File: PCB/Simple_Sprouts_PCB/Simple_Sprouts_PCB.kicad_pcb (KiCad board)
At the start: 4 copper layers, 69 x 70.6 mm, 43 parts, among them J1 Raspberry_Pi_5, J3 Soil Sensor, J4 Soil Sensor, J6 Temperature Sensor, J7 Air Quality Sensor, J8 Humidity Sensor, J9 HC-SR04, Q1 IRLB8721PbF, Q2 IRLB8721PbF, Q3 IRLB8721PbF, Q4 IRLB8721PbF, Q5 IRLB8721PbF, Q6 IRLB8721PbF

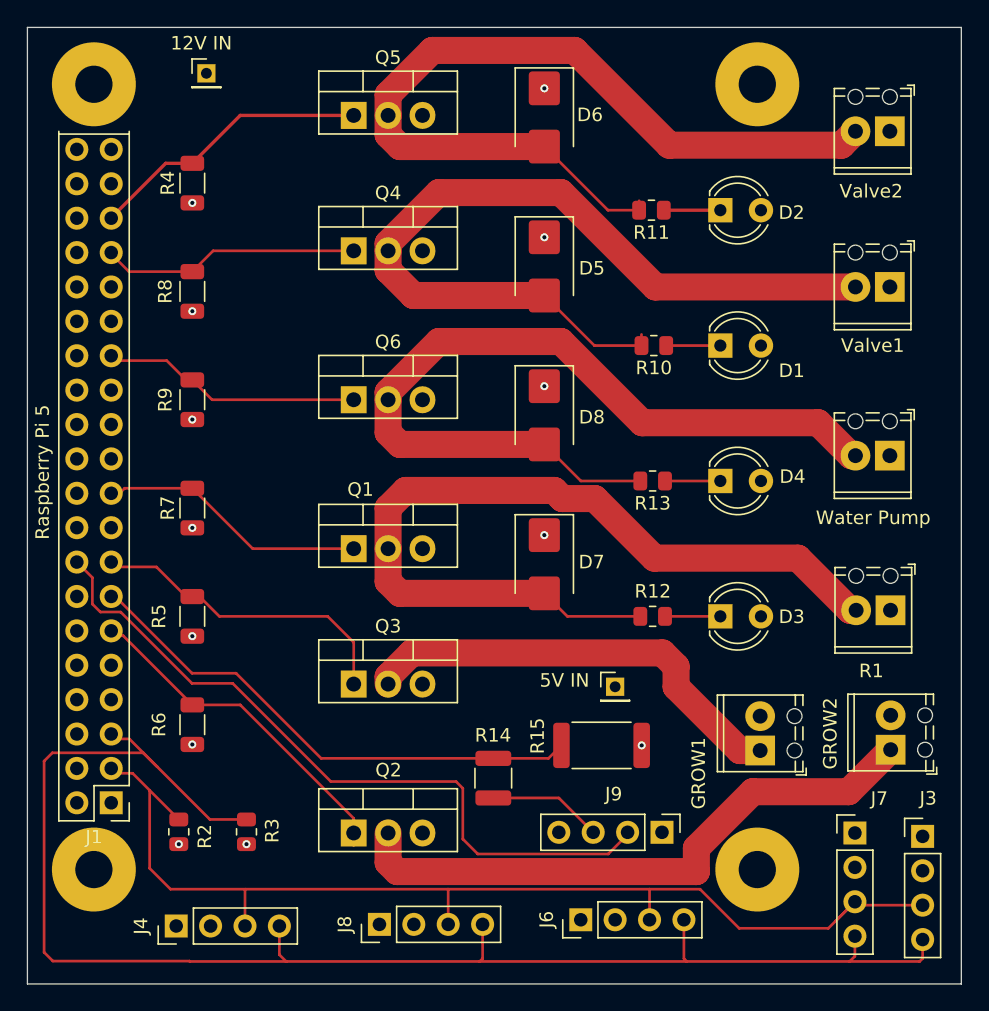
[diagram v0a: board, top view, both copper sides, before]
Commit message: Add files via upload
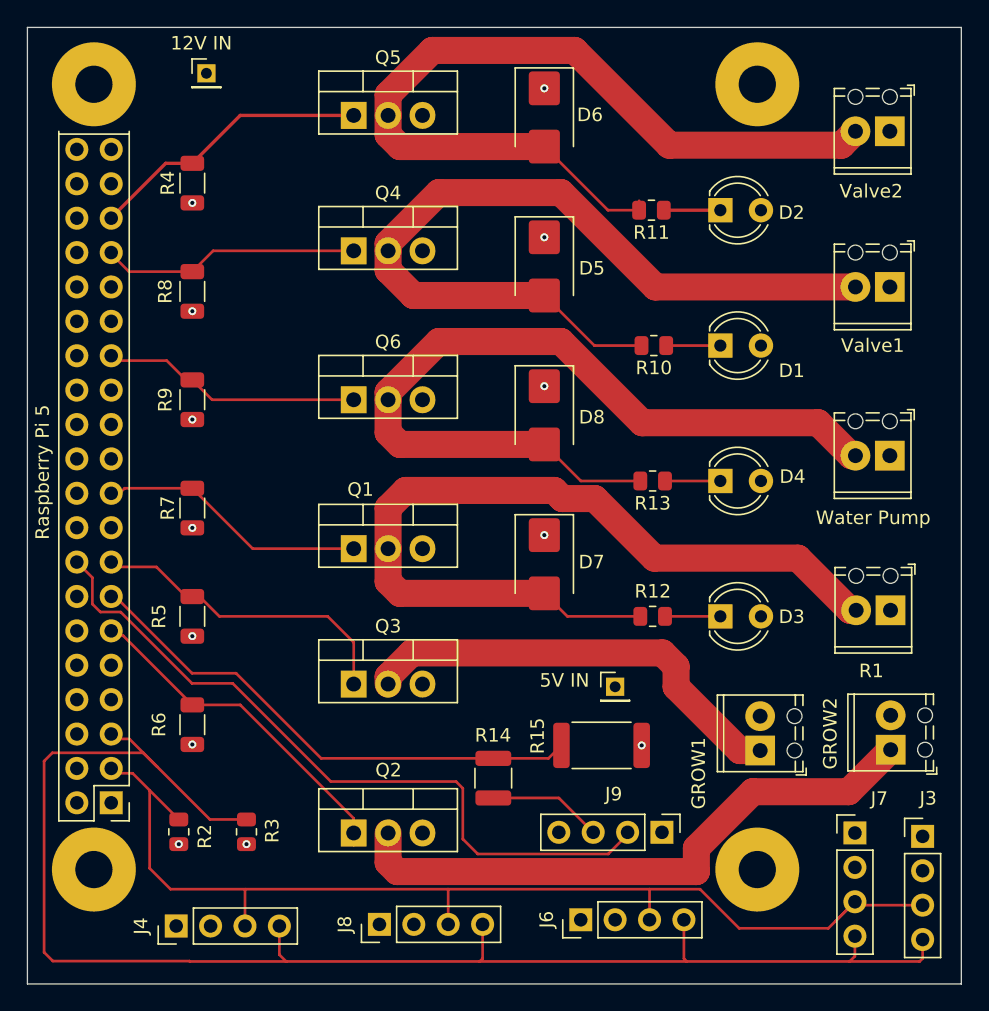
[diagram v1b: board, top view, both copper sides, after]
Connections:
- GROW1 pad 1: (no net) -> Net-(Q3-D)
- GROW1 pad 2: (no net) -> +5V
- GROW2 pad 1: (no net) -> Net-(Q2-D)
- GROW2 pad 2: (no net) -> +5V
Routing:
- net +3.3V: track 11.1 -> 34.4 mm
- net +5V: track 92.3 -> 113.9 mm
- net Net-(Q2-D): track 45.4 -> 44.3 mm
- net Net-(D5-A): track 62.8 -> 62.0 mm
- removed copper zone on In2.Cu, net +3.3V
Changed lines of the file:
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@@
 			(layers "*.Cu" "*.Mask")
 			(remove_unused_layers no)
+			(net 18 "Net-(Q3-D)")
 		)
 		(pad "2" thru_hole circle
@@
 			(layers "*.Cu" "*.Mask")
 			(remove_unused_layers no)
+			(net 11 "+5V")
 		)
 		(model "${KICAD8_3DMODEL_DIR}/TerminalBlock_Phoenix.3dshapes/TerminalBlock_Phoenix_MPT-0,5-2-2.54_1x02_P2.54mm_Horizontal.wrl"
@@
 			(at 2.11 48.25 180)
 			(layer "F.SilkS")
+			(hide yes)
 			(effects
 				(font
@@
 			(layers "*.Cu" "*.Mask")
 			(remove_unused_layers no)
+			(net 17 "Net-(Q2-D)")
 		)
 		(pad "2" thru_hole circle
@@
 			(layers "*.Cu" "*.Mask")
 			(remove_unused_layers no)
+			(net 11 "+5V")
 		)
 		(model "${KICAD8_3DMODEL_DIR}/TerminalBlock_Phoenix.3dshapes/TerminalBlock_Phoenix_MPT-0,5-2-2.54_1x02_P2.54mm_Horizontal.wrl"
@@
 	)
 	(segment
-		(start 163.445 84.3)
-		(end 163.445 83.475)
-		(width 0.2)
-		(layer "F.Cu")
-		(net 6)
-	)
-	(segment
 		(start 164.47 79.97)
 		(end 179.25 79.97)
@@
 	)
 	(segment
+		(start 119.09 120.72)
+		(end 121.74 118.07)
+		(width 1)
+		(layer "In2.Cu")
+		(net 11)
+	)
+	(segment
 		(start 159 124.5)
 		(end 163.73 124.5)
@@
 	)
 	(segment
+		(start 129.08 127.17)
+		(end 120.96 127.17)
+		(width 1)
+		(layer "In2.Cu")
+		(net 11)
+	)
+	(segment
 		(start 179.74 109.5)
 		(end 181.85 111.61)
@@
 	)
 	(segment
+		(start 119.09 125.3)
+		(end 119.09 120.72)
+		(width 1)
+		(layer "In2.Cu")
+		(net 11)
+	)
+	(segment
 		(start 158.96 126.71)
 		(end 156.17 129.5)
@@
 	)
 	(segment
+		(start 120.96 127.17)
+		(end 119.09 125.3)
+		(width 1)
+		(layer "In2.Cu")
+		(net 11)
+	)
+	(segment
 		(start 179.21 120.3)
 		(end 183.96 120.3)
@@
 	)
 	(segment
+		(start 121.74 118.07)
+		(end 121.74 115.53)
+		(width 1)
+		(layer "In2.Cu")
+		(net 11)
+	)
+	(segment
 		(start 164.96 123.27)
 		(end 164.96 120.42)
@@
 	)
 	(segment
-		(start 126.575 118.43)
-		(end 129.27 121.125)
+		(start 129.125 121.125)
+		(end 125.75 117.75)
+		(width 0.2)
+		(layer "In2.Cu")
+		(net 12)
+	)
+	(segment
+		(start 124.28 97.75)
+		(end 126.75 100.22)
+		(width 0.2)
+		(layer "In2.Cu")
+		(net 12)
+	)
+	(segment
+		(start 126.75 116)
+		(end 124.68 118.07)
+		(width 0.2)
+		(layer "In2.Cu")
+		(net 12)
+	)
+	(segment
+		(start 129.27 121.125)
+		(end 129.5 121.125)
 		(width 0.2)
 		(layer "In2.Cu")
@@
 	)
 	(segment
-		(start 124.54 118.43)
-		(end 126.575 118.43)
+		(start 125.75 117.75)
+		(end 124.6 117.75)
 		(width 0.2)
 		(layer "In2.Cu")
@@
 	(segment
 		(start 129.27 121.125)
+		(end 129.125 121.125)
+		(width 0.2)
+		(layer "In2.Cu")
+		(net 12)
+	)
+	(segment
+		(start 124.6 117.75)
+		(end 124.28 118.07)
+		(width 0.2)
+		(layer "In2.Cu")
+		(net 12)
+	)
+	(segment
+		(start 129.5 121.125)
 		(end 134.27 121.125)
 		(width 0.2)
@@
 	)
 	(segment
+		(start 124.68 118.07)
+		(end 124.28 118.07)
+		(width 0.2)
+		(layer "In2.Cu")
+		(net 12)
+	)
+	(segment
+		(start 126.75 100.22)
+		(end 126.75 116)
+		(width 0.2)
+		(layer "In2.Cu")
+		(net 12)
+	)
+	(segment
 		(start 134.16 124.46)
 		(end 134.17 124.45)
@@
 	)
 	(segment
-		(start 180.77 114.15)
-		(end 181.85 114.15)
-		(width 0.2)
-		(layer "F.Cu")
-		(net 17)
-	)
-	(segment
-		(start 178.75 117.25)
-		(end 181.85 114.15)
+		(start 171.668881 117.25)
+		(end 178.75 117.25)
 		(width 2)
 		(layer "F.Cu")
@@
 	)
 	(segment
-		(start 171.668881 117.25)
-		(end 178.75 117.25)
+		(start 167.5 123.15)
+		(end 167.5 121.418881)
 		(width 2)
 		(layer "F.Cu")
@@
 	)
 	(segment
-		(start 167.5 123.15)
-		(end 167.5 121.418881)
+		(start 178.75 117.25)
+		(end 181.85 114.15)
 		(width 2)
 		(layer "F.Cu")
@@
 	)
 	(segment
+		(start 170.71 114.21)
+		(end 172.21 114.21)
+		(width 2)
+		(layer "F.Cu")
+		(net 18)
+	)
+	(segment
 		(start 165 107)
 		(end 166 108)
@@
 	)
 	(segment
-		(start 170.71 114.21)
-		(end 172.21 114.21)
-		(width 2)
-		(layer "F.Cu")
-		(net 18)
-	)
-	(segment
 		(start 129.8075 86.8375)
 		(end 128.38 85.41)
@@
 		(polygon
 			(pts
-				(xy 122.5 117) (xy 122.5 119.5) (xy 119.53 119.49) (xy 119.53 126.49) (xy 126 126.5) (xy 126 125)
+				(xy 122.5 114.5) (xy 122.5 119.5) (xy 119.53 119.49) (xy 119.53 126.49) (xy 126 126.5) (xy 126 125)
 				(xy 156 125) (xy 156 123) (xy 163.22 123.02) (xy 163.22 114.02) (xy 167.5 114) (xy 167.5 108.5)
-				(xy 186 108.5) (xy 186 130.5) (xy 118.81 130.44) (xy 118.81 116.94)
-			)
-		)
-	)
-	(zone
-		(net 12)
-		(net_name "+3.3V")
-		(layer "In2.Cu")
-		(hatch edge 0.5)
-		(priority 1)
-		(connect_pads
-			(clearance 0.5)
-		)
-		(min_thickness 0.25)
-		(filled_areas_thickness no)
-		(fill yes
-			(thermal_gap 0.5)
-			(thermal_bridge_width 0.5)
-			(smoothing chamfer)
-		)
-		(polygon
-			(pts
-				(xy 137.2 124.4) (xy 137.27 117.3) (xy 123.27 117.3) (xy 123.47 124.3)
+				(xy 186 108.5) (xy 186 130.5) (xy 118.81 130.44) (xy 118.81 114.44)
 			)
 		)
